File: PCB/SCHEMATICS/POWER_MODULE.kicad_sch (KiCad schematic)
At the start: 44 parts, among them Q1 PMOS, U1 C7433, U2 AMS1117-3.3, U4 AMS1117-3.3

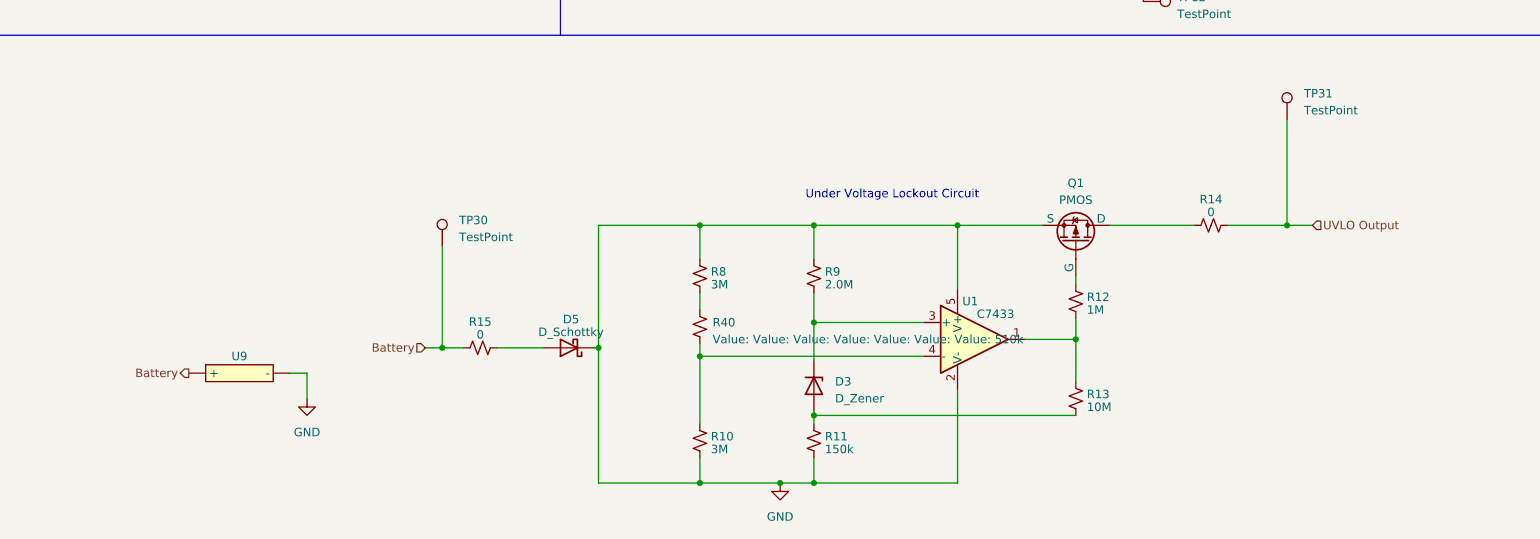
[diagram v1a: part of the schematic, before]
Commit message: Updated schematics
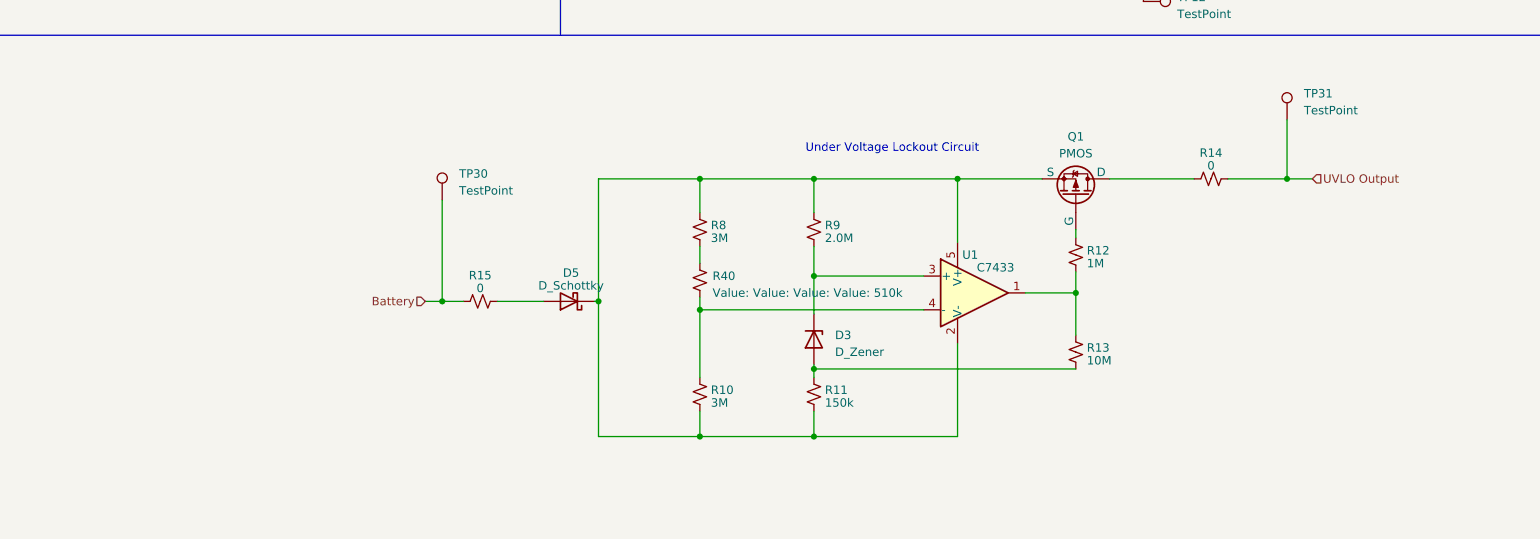
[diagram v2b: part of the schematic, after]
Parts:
- removed U9: ~, footprints:18650_Holder_SMD, symbol Battery holder:18650_holder
- Q1: footprint (none) -> footprint:SOT-23-3_L3.0-W1.6-P1.90-LS2.8-BR; PART  C20917 -> C2959854; Unit Price 0.0864 -> 0.0851
- R1, R14, R15, R4, R5, R7: PART  C17168 -> C17168
- R12: footprint (none) -> footprint:R1206
- R40: value Value: Value: Value: Value: Value: Value: 510k -> Value: Value: Value: 510k; footprint (none) -> footprint:R0402
- TP4054-42-SOT25R: footprint LIB_TP4054-42-SOT25-R:SOT95P280X100-5N -> footprint:SOT-23-5_L3.0-W1.7-P0.95-LS2.8-BL
- U1: footprint Package_TO_SOT_SMD:TSOT-23-5 -> footprint:SOIC-8_L4.9-W3.9-P1.27-LS6.0-BL
- U2, U4: footprint LIB_AMS1117-3.3:SOT229P700X180-4N -> footprint:SOT-223-4_L6.5-W3.5-P2.30-LS7.0-BR; PART  U2 -> C369933; Unit Price 0.0627 -> 0.0646
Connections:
- net GND: no longer D5.1 (K), Q1.3 (S), R10.2, R11.2, R8.1, R9.1, U1.2 (V-), U1.5 (V+)
- new net: D5.1 (K), Q1.3 (S), R10.2, R11.2, R8.1, R9.1, U1.2 (V-), U1.5 (V+)
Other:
- moved on the sheet: D3, D5, Q1, R10, R11, R12, R13, R14, R15, R40, R8, R9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
